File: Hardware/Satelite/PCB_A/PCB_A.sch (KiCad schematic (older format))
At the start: 33 parts, among them J1 Batería LiPo (Soldada), J2 CONUFL001-SMD, J3 Servo Globo, J4 Conector_PCB_A-B, J5 Servo Paracaídas, M1 Spacer, M2 Spacer, M3 Spacer, Q1 SSM3J338R,LF, Q2 BC817, U4 AP9211SA-AF-HAC-7

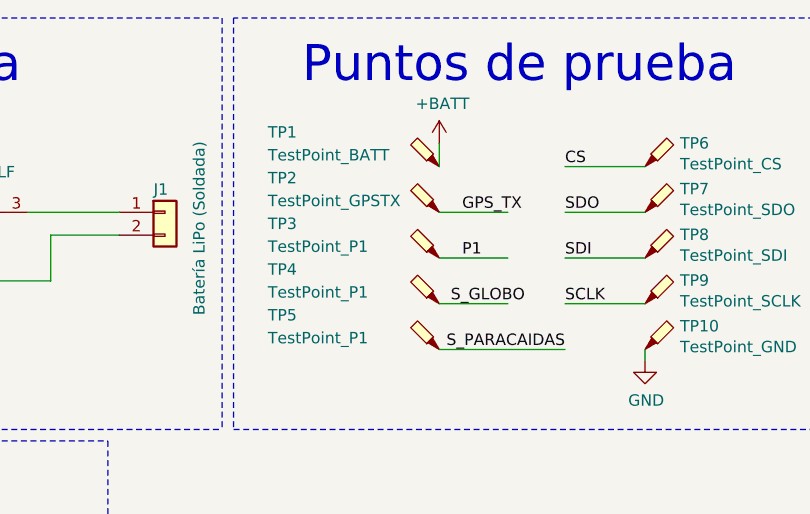
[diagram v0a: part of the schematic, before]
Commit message: Completado nuevo PCB_A
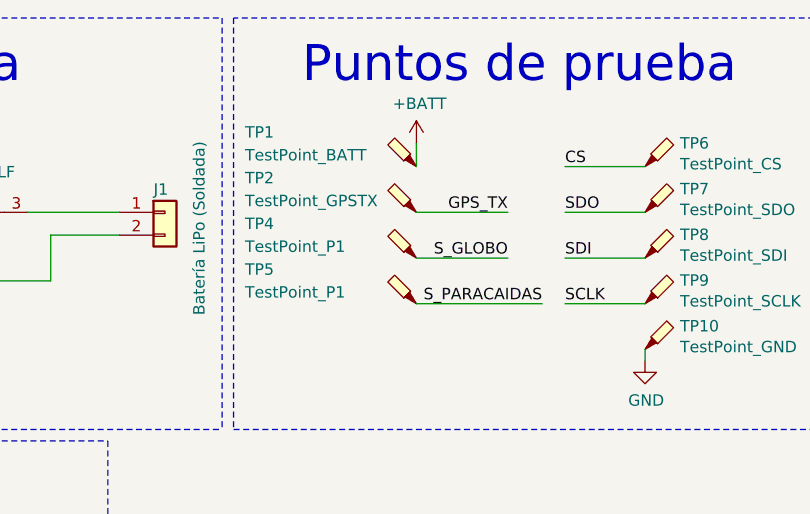
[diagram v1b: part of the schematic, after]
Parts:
- removed TP3: TestPoint_P1, TestPoint:TestPoint_Pad_D1.0mm, symbol Connector:TestPoint_Probe
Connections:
- wire segments 93 -> 92
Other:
- moved on the sheet: TP1, TP2, TP4, TP5
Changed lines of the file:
@@
 L power:+BATT #PWR014
 U 1 1 5C2D3F1A
-P 5050 1100
-F 0 "#PWR014" H 5050 950 50  0001 C CNN
-F 1 "+BATT" H 5064 1275 50  0000 C CNN
-F 2 "" H 5050 1100 50  0001 C CNN
-F 3 "" H 5050 1100 50  0001 C CNN
-	1    5050 1100
+P 4950 1100
+F 0 "#PWR014" H 4950 950 50  0001 C CNN
+F 1 "+BATT" H 4964 1275 50  0000 C CNN
+F 2 "" H 4950 1100 50  0001 C CNN
+F 3 "" H 4950 1100 50  0001 C CNN
+	1    4950 1100
 	1    0    0    -1
 $EndComp
@@
 L Connector:TestPoint_Probe TP2
 U 1 1 5C2DEC1A
-P 5050 1400
-F 0 "TP2" H 5800 1550 50  0000 R CNN
-F 1 "TestPoint_GPSTX" H 5800 1450 50  0000 R CNN
-F 2 "TestPoint:TestPoint_Pad_D1.0mm" H 5250 1400 50  0001 C CNN
-F 3 "~" H 5250 1400 50  0001 C CNN
-	1    5050 1400
+P 4950 1400
+F 0 "TP2" H 5700 1550 50  0000 R CNN
+F 1 "TestPoint_GPSTX" H 5700 1450 50  0000 R CNN
+F 2 "TestPoint:TestPoint_Pad_D1.0mm" H 5150 1400 50  0001 C CNN
+F 3 "~" H 5150 1400 50  0001 C CNN
+	1    4950 1400
 	-1   0    0    -1
 $EndComp
 Wire Wire Line
-	5050 1400 5350 1400
-Text Label 5150 1400 0    50   ~ 0
+	4950 1400 5350 1400
+Text Label 5350 1400 2    50   ~ 0
 GPS_TX
 $Comp
-L Connector:TestPoint_Probe TP3
-U 1 1 5C2E59E7
-P 5050 1600
-F 0 "TP3" H 5800 1750 50  0000 R CNN
-F 1 "TestPoint_P1" H 5800 1650 50  0000 R CNN
-F 2 "TestPoint:TestPoint_Pad_D1.0mm" H 5250 1600 50  0001 C CNN
-F 3 "~" H 5250 1600 50  0001 C CNN
-	1    5050 1600
+L Connector:TestPoint_Probe TP4
+U 1 1 5C2E7A24
+P 4950 1600
+F 0 "TP4" H 5700 1750 50  0000 R CNN
+F 1 "TestPoint_P1" H 5700 1650 50  0000 R CNN
+F 2 "TestPoint:TestPoint_Pad_D1.0mm" H 5150 1600 50  0001 C CNN
+F 3 "~" H 5150 1600 50  0001 C CNN
+	1    4950 1600
 	-1   0    0    -1
 $EndComp
 Wire Wire Line
-	5050 1600 5350 1600
-Text Label 5150 1600 0    50   ~ 0
-P1
-$Comp
-L Connector:TestPoint_Probe TP4
-U 1 1 5C2E7A24
-P 5050 1800
-F 0 "TP4" H 5800 1950 50  0000 R CNN
-F 1 "TestPoint_P1" H 5800 1850 50  0000 R CNN
-F 2 "TestPoint:TestPoint_Pad_D1.0mm" H 5250 1800 50  0001 C CNN
-F 3 "~" H 5250 1800 50  0001 C CNN
-	1    5050 1800
-	-1   0    0    -1
-$EndComp
-Wire Wire Line
-	5050 1800 5350 1800
+	4950 1600 5350 1600
 $Comp
 L Connector:TestPoint_Probe TP5
 U 1 1 5C2E94B0
-P 5050 2000
-F 0 "TP5" H 5800 2150 50  0000 R CNN
-F 1 "TestPoint_P1" H 5800 2050 50  0000 R CNN
-F 2 "TestPoint:TestPoint_Pad_D1.0mm" H 5250 2000 50  0001 C CNN
-F 3 "~" H 5250 2000 50  0001 C CNN
-	1    5050 2000
+P 4950 1800
+F 0 "TP5" H 5700 1950 50  0000 R CNN
+F 1 "TestPoint_P1" H 5700 1850 50  0000 R CNN
+F 2 "TestPoint:TestPoint_Pad_D1.0mm" H 5150 1800 50  0001 C CNN
+F 3 "~" H 5150 1800 50  0001 C CNN
+	1    4950 1800
 	-1   0    0    -1
 $EndComp
-Text Label 5100 1800 0    50   ~ 0
+Text Label 5350 1600 2    50   ~ 0
 S_GLOBO
-Text Label 5600 2000 2    50   ~ 0
+Text Label 5500 1800 2    50   ~ 0
 S_PARACAIDAS
 Wire Wire Line
-	5050 2000 5600 2000
+	4950 1800 5500 1800
 Wire Wire Line
 	5950 2050 5950 2000
 Wire Wire Line
-	5050 1100 5050 1200
+	4950 1100 4950 1200
 $Comp
 L Connector:TestPoint_Probe TP1
 U 1 1 5C2FCED2
-P 5050 1200
-F 0 "TP1" H 5800 1350 50  0000 R CNN
-F 1 "TestPoint_BATT" H 5800 1250 50  0000 R CNN
-F 2 "TestPoint:TestPoint_Pad_D1.0mm" H 5250 1200 50  0001 C CNN
-F 3 "~" H 5250 1200 50  0001 C CNN
-	1    5050 1200
+P 4950 1200
+F 0 "TP1" H 5700 1350 50  0000 R CNN
+F 1 "TestPoint_BATT" H 5700 1250 50  0000 R CNN
+F 2 "TestPoint:TestPoint_Pad_D1.0mm" H 5150 1200 50  0001 C CNN
+F 3 "~" H 5150 1200 50  0001 C CNN
+	1    4950 1200
 	-1   0    0    -1
 $EndComp
